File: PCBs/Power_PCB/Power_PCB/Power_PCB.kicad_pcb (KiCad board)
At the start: 4 copper layers, 100 x 120 mm, 94 parts, among them IC1 ADS1115BQDGSRQ1, IC10 ACS712ELCTR-20A-T, IC2 ADS1115BQDGSRQ1, IC3 W25Q16JVUXIQ_TR, IC7 ACS712ELCTR-20A-T, IC8 ACS712ELCTR-20A-T, IC9 ACS712ELCTR-20A-T, J1 Conn_01x02, J10 Conn_01x04, J11 Conn_01x04, J12 Conn_01x04, J13 Conn_01x04, J14 Conn_01x04, J16 Conn_01x02, J17 Conn_01x02, J19 Conn_01x02, J2 Conn_01x02, J20 Conn_01x02, J3 Conn_01x02, J4 Conn_01x02, J5 Conn_01x02, J6 Conn_01x02, J7 USB_C_Receptacle_USB2.0_16P, J8 Conn_01x02, Q1 SUD45P03-09, Q2 RQ6E080AJ, Q3 RQ6E080AJ, SW1 SW_Push_Open, SW2 SW_Push, SW3 SW_Push, U1 ESP32-S3, U2 AMS1117-3.3, U3 USBLC6-2SC6, U5 TVS3300DRV, Y1 Crystal_GND24

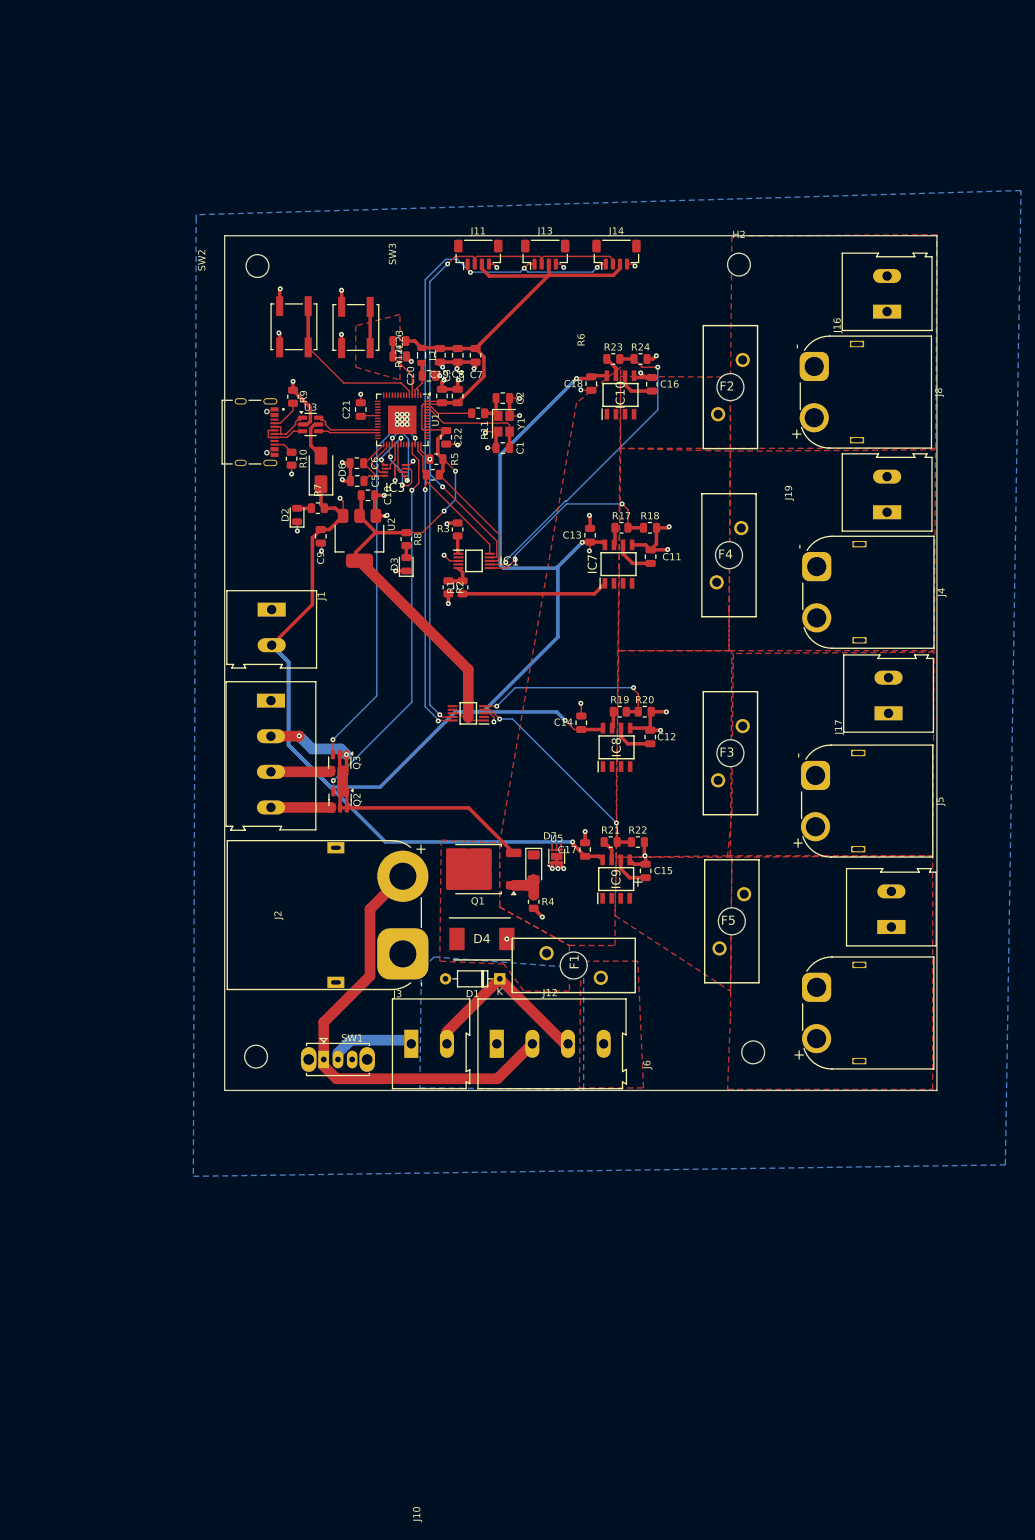
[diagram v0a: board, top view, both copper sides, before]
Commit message: Second iteration power board
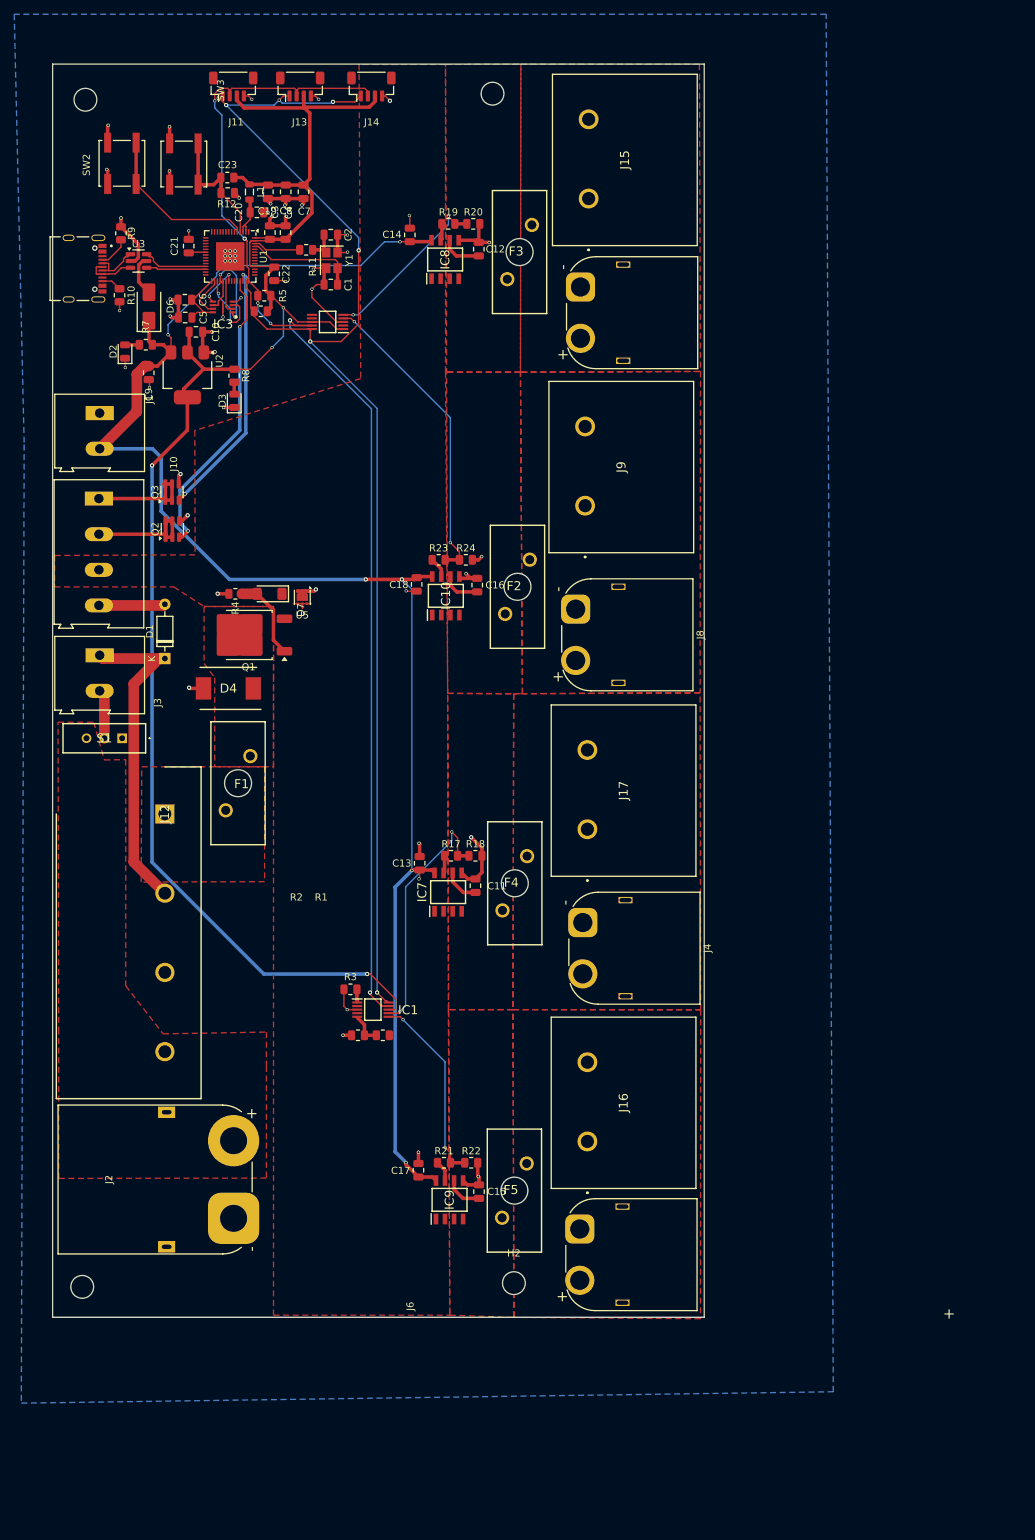
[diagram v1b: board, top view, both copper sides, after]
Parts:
- removed J19, J20: Conn_01x02, TerminalBlock:TerminalBlock_Altech_AK300-2_P5.00mm
- removed SW1: SW_Push_Open, Button_Switch_THT:SW_Slide_SPDT_Straight_CK_OS102011MS2Q
- added J15: 8PCV-02-006, iprl_footprints:8PCV02006, F.Cu at (128.5, 33.7)
- added J9: 8PCV-02-006, iprl_footprints:8PCV02006, F.Cu at (128.0, 76.8)
- added S1: SLW-116641-5A-S-D, iprl_footprints:SLW1166415ASD, F.Cu at (63.0, 109.5)
- J12: value Conn_01x04 -> 8PCV-04-006; footprint TerminalBlock:TerminalBlock_Altech_AK300-4_P5.00mm -> iprl_footprints:SHDR4W114P0X1112_1X4_4628X2032X1956P
- J16, J17: value Conn_01x02 -> 8PCV-02-006; footprint TerminalBlock:TerminalBlock_Altech_AK300-2_P5.00mm -> iprl_footprints:8PCV02006
- moved H2 146.4 mm to (118.0, 186.0)
- moved H4 139.5 mm to (115.0, 19.0)
- moved J16 123.9 mm to (128.3, 166.1)
- moved F3 76.3 mm to (118.8, 41.2)
- moved J5 76.1 mm to (127.3, 46.1)
- moved C12 72.6 mm to (113.1, 40.8)
- moved R19 72.6 mm to (108.8, 37.3)
- moved R20 72.6 mm to (112.3, 37.3)
- moved C14 72.6 mm to (103.4, 38.8)
- moved IC8 72.6 mm to (108.3, 42.3)
- moved J3 69.9 mm to (59.8, 97.8), turned to -90 degrees
- moved R3 66.3 mm to (95.0, 144.8), turned to 0 degrees
- moved D1 65.1 mm to (69.0, 98.3), turned to 90 degrees
- moved IC1 64.6 mm to (98.2, 147.6)
- moved R2 64.2 mm to (96.1, 151.2), turned to 180 degrees
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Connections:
- IC1 pad 6: /Current_sensing/DRILL_READ -> /Current_sensing/COMMS_READ
- IC1 pad 7: /Current_sensing/ARM_READ -> /Current_sensing/DRILL_READ
- IC2 pad 4: /Current_sensing/COMMS_READ -> /Current_sensing/ARM_READ
- J10 pad 1: GND -> Net-(J10-Pin_1)
- J10 pad 2: /14V8_PROTECTED -> Net-(J10-Pin_2)
- J10 pad 3: Net-(J10-Pin_3) -> /14V8_PROTECTED
- J10 pad 4: Net-(J10-Pin_4) -> GND
- J12 pad 1: GND -> /Power/RELAY_OUT
- J12 pad 2: /Power/14V8_IN -> /Power/EMERG_OUT
- J12 pad 3: /Power/EMERG_OUT -> GND
- J12 pad 4: /Power/RELAY_OUT -> /Power/14V8_IN
- J16 pad 2: /Connectors/14V8_ARM_OUT -> /Connectors/14V8_COMMS_OUT
- J17 pad 2: /Connectors/14V8_DRIVE_OUT -> /Connectors/14V8_DRILL_OUT
- J3 pad 1: Net-(J3-Pin_1) -> /Power/EMERG_OUT
- J3 pad 2: /Power/EMERG_OUT -> Net-(J3-Pin_2)
- Q2 pad 1: /14V8_PROTECTED -> Net-(J10-Pin_2)
- Q2 pad 2: /14V8_PROTECTED -> Net-(J10-Pin_2)
- Q2 pad 4: Net-(J10-Pin_4) -> GND
- Q2 pad 5: /14V8_PROTECTED -> Net-(J10-Pin_2)
- Q2 pad 6: /14V8_PROTECTED -> Net-(J10-Pin_2)
- Q3 pad 1: /14V8_PROTECTED -> Net-(J10-Pin_1)
- Q3 pad 2: /14V8_PROTECTED -> Net-(J10-Pin_1)
- Q3 pad 4: Net-(J10-Pin_3) -> GND
- Q3 pad 5: /14V8_PROTECTED -> Net-(J10-Pin_1)
- Q3 pad 6: /14V8_PROTECTED -> Net-(J10-Pin_1)
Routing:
- net /14V8_PROTECTED: track 78.6 -> 3.28 mm, vias 2 -> 0
- net +3.3V: track 161.4 -> 229.2 mm, vias 2 -> 4
- net /SCL: track 118.1 -> 182.8 mm, vias 5 -> 6
- net /Power/14V8_IN: track 63.3 -> 0.00 mm
- net /SDA: track 114.6 -> 172.2 mm, vias 4 -> 6
- net +5V: track 246.8 -> 224.8 mm, vias 6 -> 7
- net /Power/EMERG_OUT: track 25.6 -> 46.9 mm
- net GND: track 119.8 -> 137.8 mm, vias 60 -> 56
- net Net-(J10-Pin_2): track 0.00 -> 17.7 mm
- net /IND_YELLOW: track 53.4 -> 36.6 mm
- net Net-(J10-Pin_1): track 0.00 -> 16.1 mm
- net /IND_GREEN: track 54.2 -> 41.5 mm
- net Net-(J3-Pin_1): track 12.2 -> 0.00 mm
- net Net-(J10-Pin_4): track 8.48 -> 0.00 mm
- net Net-(J10-Pin_3): track 8.41 -> 0.00 mm
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- added copper zone on In1.Cu, net /14V8_ARM_OUT
- added copper zone on In2.Cu, net /14V8_ARM_OUT
- added copper zone on In1.Cu, net /14V8_COMMS_OUT
- added copper zone on In2.Cu, net /14V8_COMMS_OUT
- added copper zone on In1.Cu, net /14V8_DRILL_OUT
- added copper zone on In2.Cu, net /14V8_DRILL_OUT
- added copper zone on In1.Cu, net /14V8_DRIVE_OUT
- added copper zone on In2.Cu, net /14V8_DRIVE_OUT
- added copper zone on In1.Cu, net /14V8_PROTECTED
- added copper zone on In2.Cu, net /14V8_PROTECTED
- added copper zone on In1.Cu, net /Connectors/14V8_ARM_OUT
- added copper zone on In2.Cu, net /Connectors/14V8_ARM_OUT
- added copper zone on In1.Cu, net /Connectors/14V8_COMMS_OUT
- added copper zone on In2.Cu, net /Connectors/14V8_COMMS_OUT
- added copper zone on In1.Cu, net /Connectors/14V8_DRILL_OUT
- added copper zone on In2.Cu, net /Connectors/14V8_DRILL_OUT
- added copper zone on In1.Cu, net /Connectors/14V8_DRIVE_OUT
- added copper zone on In2.Cu, net /Connectors/14V8_DRIVE_OUT
- added copper zone on F.Cu, net /Power/14V8_IN
- added copper zone on In1.Cu, net /Power/14V8_IN
- added copper zone on In2.Cu, net /Power/14V8_IN
- added copper zone on In1.Cu, net /Power/PROTEC_IN
- added copper zone on In2.Cu, net /Power/PROTEC_IN
- added copper zone on In1.Cu, net /Power/RELAY_OUT
- added copper zone on In2.Cu, net /Power/RELAY_OUT
- removed copper zone on B.Cu, net /Power/EMERG_OUT
- removed copper zone on F.Cu, net /RESET
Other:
- board size 100 x 120 mm -> 91.5 x 175.9 mm

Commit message: Power board revisions
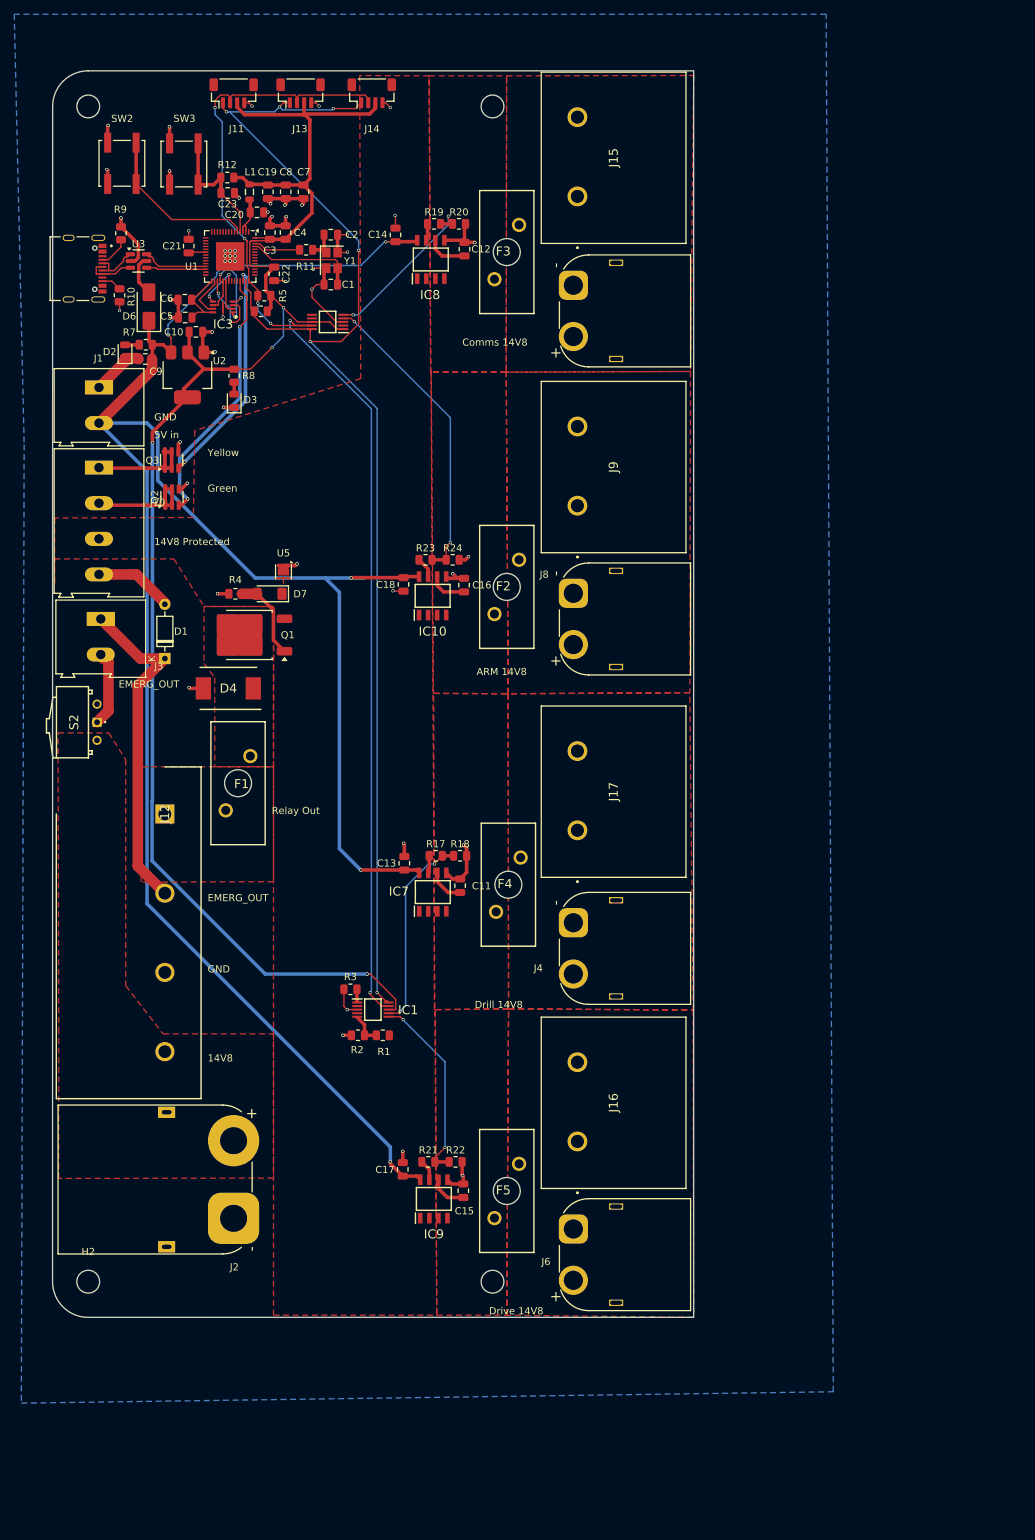
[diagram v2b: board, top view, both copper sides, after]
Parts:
- removed S1: SLW-116641-5A-S-D, iprl_footprints:SLW1166415ASD
- added S2: EGJ1210AAT2, iprl_footprints:EGJ1210AAT2, F.Cu at (59.5, 107.2)
- moved H2 59.8 mm to (58.2, 185.8)
- moved H3 57.6 mm to (115.0, 185.8)
- moved H1 57.2 mm to (115.0, 20.8)
- moved H4 56.8 mm to (58.2, 20.8)
- moved J3 5.10 mm to (60.0, 92.8)
- moved Q2 4.50 mm to (70.0, 75.6)
- moved Q3 4.50 mm to (70.0, 70.4)
- moved U5 4.45 mm to (85.7, 86.1)
- moved J10 4.35 mm to (59.8, 71.5)
- moved J1 3.60 mm to (59.8, 60.2)
- moved J8 2.25 mm to (126.3, 89.2)
- moved IC9 2.20 mm to (106.8, 174.2)
- moved R21 2.20 mm to (106.0, 169.0)
- moved R22 2.20 mm to (109.8, 169.0)
- moved C15 2.20 mm to (110.9, 173.0)
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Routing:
- net +5V: track 224.8 -> 304.2 mm, vias 7 -> 5
- net /Current_sensing/DRILL_READ: track 35.2 -> 28.1 mm
- net GND: track 137.8 -> 143.2 mm, vias 56 -> 54
- net /IND_GREEN: track 41.5 -> 37.1 mm
- net /IND_YELLOW: track 36.6 -> 32.2 mm
- net Net-(J3-Pin_2): track 6.92 -> 11.1 mm
- net /Current_sensing/DRIVE_READ: track 25.9 -> 24.2 mm
- net +3.3V: track 229.2 -> 228.0 mm
- net /SDA: track 172.2 -> 171.3 mm
- net /SCL: track 182.8 -> 182.1 mm
- removed copper zone on In2.Cu, net /14V8_ARM_OUT
- removed copper zone on In2.Cu, net /14V8_COMMS_OUT
- removed copper zone on In2.Cu, net /14V8_DRILL_OUT
- removed copper zone on In2.Cu, net /14V8_DRIVE_OUT
- removed copper zone on In2.Cu, net /14V8_PROTECTED
- removed copper zone on In2.Cu, net /Connectors/14V8_ARM_OUT
- removed copper zone on In2.Cu, net /Connectors/14V8_COMMS_OUT
- removed copper zone on In2.Cu, net /Connectors/14V8_DRILL_OUT
- removed copper zone on In2.Cu, net /Connectors/14V8_DRIVE_OUT
- removed copper zone on In2.Cu, net /Power/14V8_IN
- removed copper zone on In2.Cu, net /Power/PROTEC_IN
- removed copper zone on In2.Cu, net /Power/RELAY_OUT
- removed copper zone on In1.Cu, net GND
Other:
- board size 91.5 x 175.9 mm -> 90 x 175 mm
- board text added: "14V8"
- board text added: "14V8 Protected"
- board text added: "5V in"
- board text added: "ARM 14V8"
- board text added: "Comms 14V8"
- board text added: "Drill 14V8"
- board text added: "Drive 14V8"
- board text added: "EMERG_OUT"
- board text added: "GND"
- board text added: "Green"
- board text added: "Relay Out"
- board text added: "Yellow"
